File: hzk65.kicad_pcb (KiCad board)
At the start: 2 copper layers, 314.3 x 100 mm, 136 parts, among them SW1 SW_Push, SW10 SW_Push, SW11 SW_Push, SW12 SW_Push, SW13 SW_Push, SW14 SW_Push, SW16 SW_Push, SW17 SW_Push, SW18 SW_Push, SW19 SW_Push, SW2 SW_Push, SW20 SW_Push, SW21 SW_Push, SW22 SW_Push, SW23 SW_Push, SW24 SW_Push, SW25 SW_Push, SW26 SW_Push, SW27 SW_Push, SW28 SW_Push, SW29 SW_Push, SW3 SW_Push, SW31 SW_Push, SW32 SW_Push, SW33 SW_Push, SW34 SW_Push, SW35 SW_Push, SW36 SW_Push, SW37 SW_Push, SW38 SW_Push, SW39 SW_Push, SW4 SW_Push, SW40 SW_Push, SW41 SW_Push, SW42 SW_Push, SW44 SW_Push, SW46 SW_Push, SW48 SW_Push, SW49 SW_Push, SW5 SW_Push, SW50 SW_Push, SW51 SW_Push, SW52 SW_Push, SW53 SW_Push, SW54 SW_Push, SW55 SW_Push, SW56 SW_Push, SW57 SW_Push, SW58 SW_Push, SW59 SW_Push, SW6 SW_Push, SW60 SW_Push, SW61 SW_Push, SW62 SW_Push, SW63 SW_Push, SW67 SW_Push, SW7 SW_Push, SW70 SW_Push, SW71 SW_Push, SW72 SW_Push, SW73 SW_Push, SW74 SW_Push, SW75 SW_Push, SW8 SW_Push, SW9 SW_Push

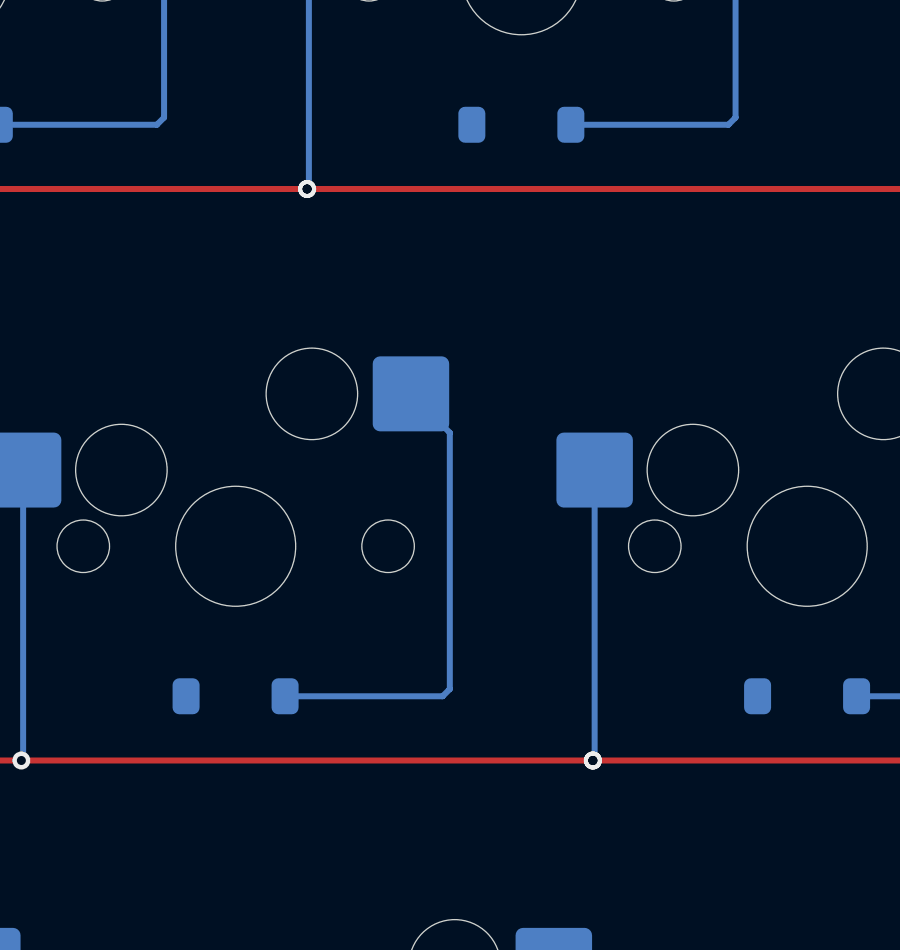
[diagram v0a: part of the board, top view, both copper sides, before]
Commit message: Fix drc via and silkscreen warnings
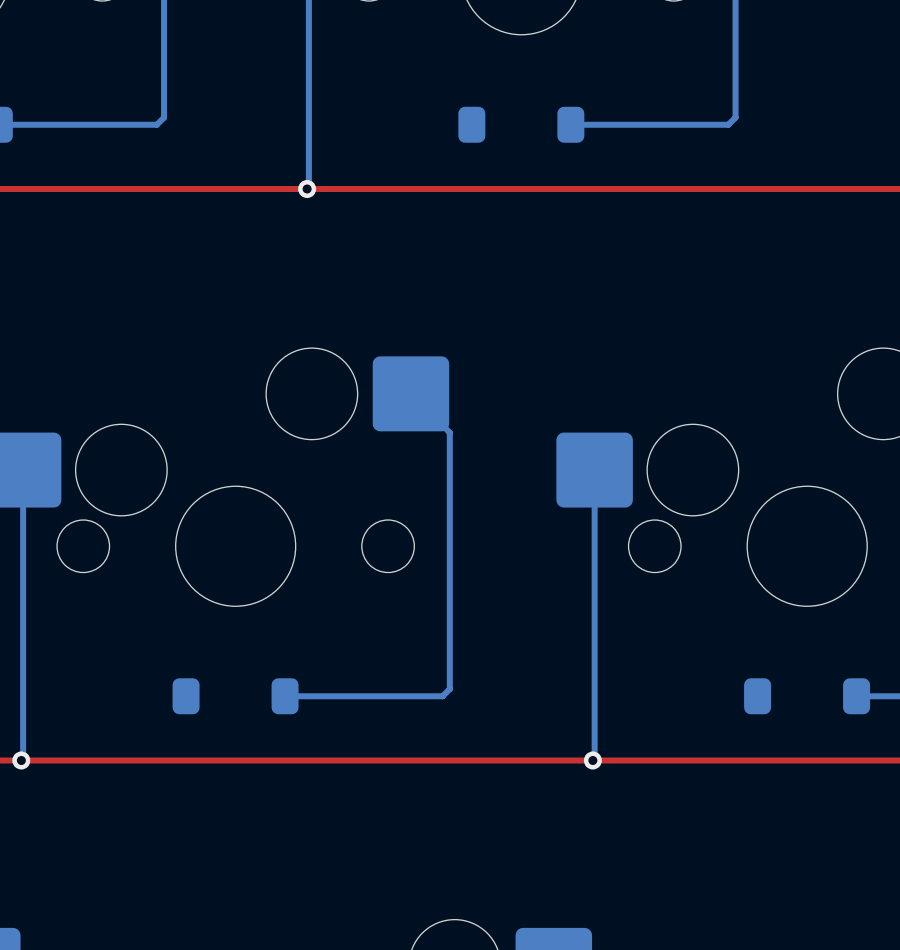
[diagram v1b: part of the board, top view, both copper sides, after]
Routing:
- net /ROW1: vias 15 -> 14
- net /ROW0: vias 15 -> 14
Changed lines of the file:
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@@
-	)
-	(via
-		(at 283.3747 116.681348)
-		(size 0.6)
-		(drill 0.3)
-		(layers "F.Cu" "B.Cu")
-		(net "/ROW0")
 	)
 	(via
@@
 		(size 0.6)
 		(drill 0.3)
-		(layers "F.Cu" "B.Cu")
-		(net "/ROW1")
-	)
-	(via
-		(at 292.8999 135.731364)
-		(size 0.6)
-		(drill 0.3)
